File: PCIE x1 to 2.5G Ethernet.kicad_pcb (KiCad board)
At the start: 4 copper layers, 73.3 x 68.9 mm, 48 parts, among them J1 PCIexpress_bracket, J2 PCIexpress_x1, U1 RTL8125BG-CG, U2 TPS62590DRVT, Y1 25Mhz

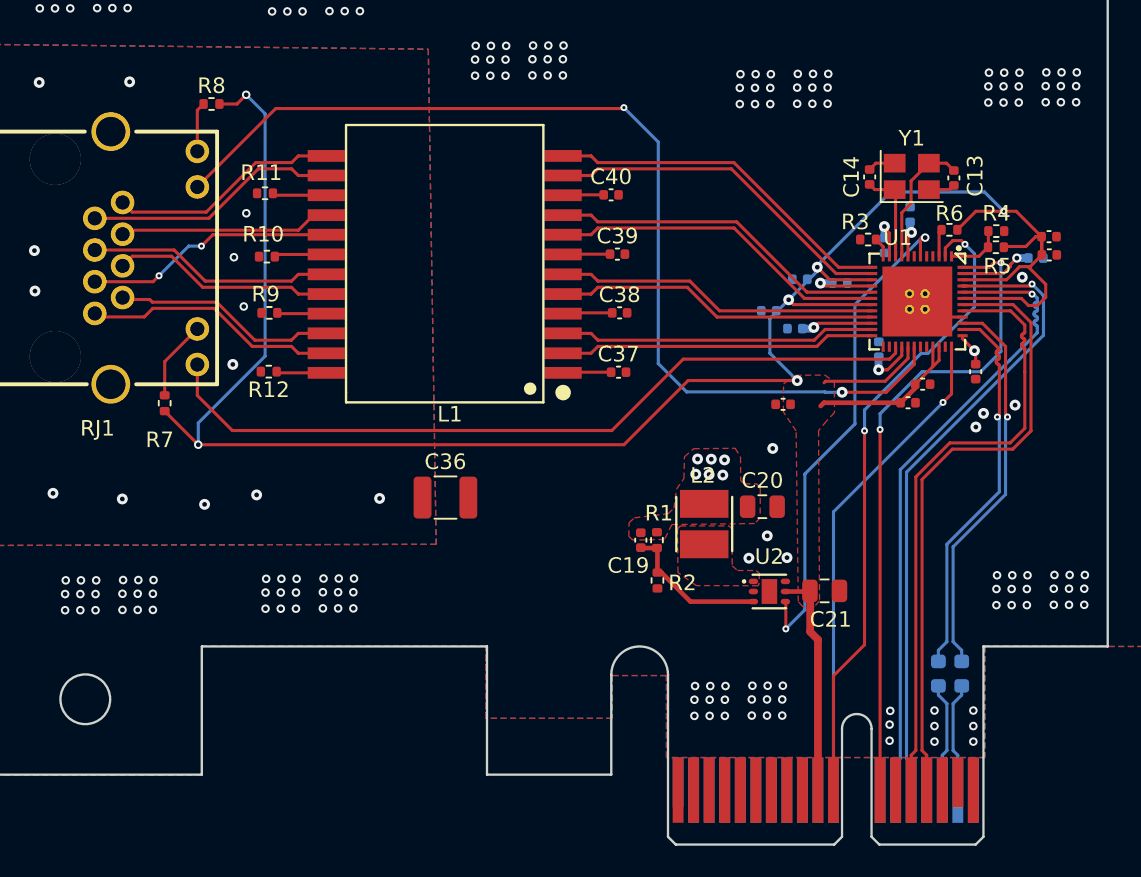
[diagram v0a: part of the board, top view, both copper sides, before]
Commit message: .
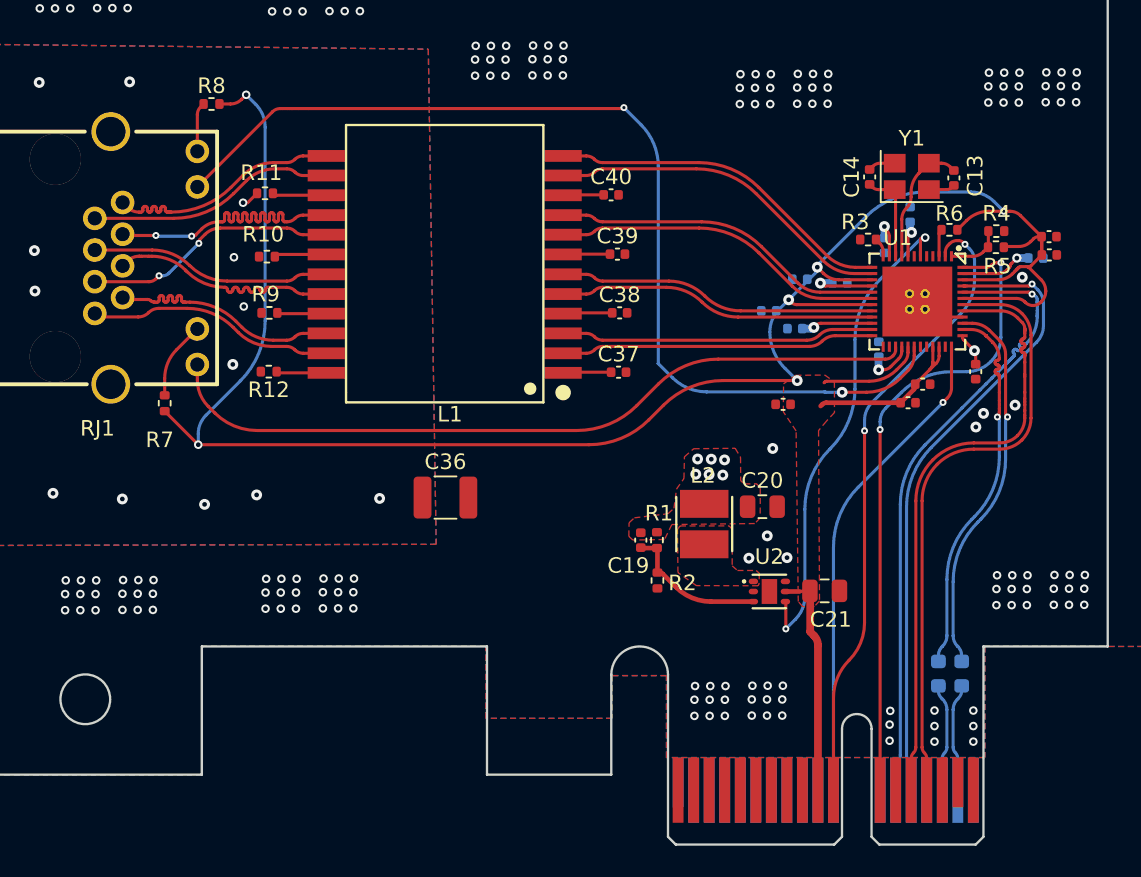
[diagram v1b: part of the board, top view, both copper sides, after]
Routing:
- net MD2+: track 13.6 -> 21.3 mm, vias 0 -> 2
- net +3.3VA: track 162.2 -> 159.9 mm
- net MD4+: track 14.4 -> 15.8 mm
- net ETH_GND: track 0.00 -> 1.15 mm
- net MD3-: track 14.4 -> 15.4 mm
- net MD1+: track 14.9 -> 15.9 mm
- net WAKE: track 41.5 -> 40.6 mm
- net REG_EN: track 32.2 -> 31.3 mm
- net LED1: track 50.3 -> 49.5 mm
- net PER0-: track 25.4 -> 24.6 mm
- net PET0-: track 40.3 -> 39.5 mm
- net LED0: track 66.1 -> 65.5 mm
- net REFCLK-: track 41.3 -> 40.7 mm
- net PER0+: track 25.1 -> 24.6 mm
- net PET0+: track 40.0 -> 39.5 mm
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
